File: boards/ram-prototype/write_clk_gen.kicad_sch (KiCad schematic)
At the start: 24 parts, among them U1 74LVC1G00, U2 74LVC1G00, U3 74LVC1G00, U4 74LVC1G00, U5 74LVC1G00, U6 74LVC1G00, U7 74LVC1G00, U8 74LVC1G00

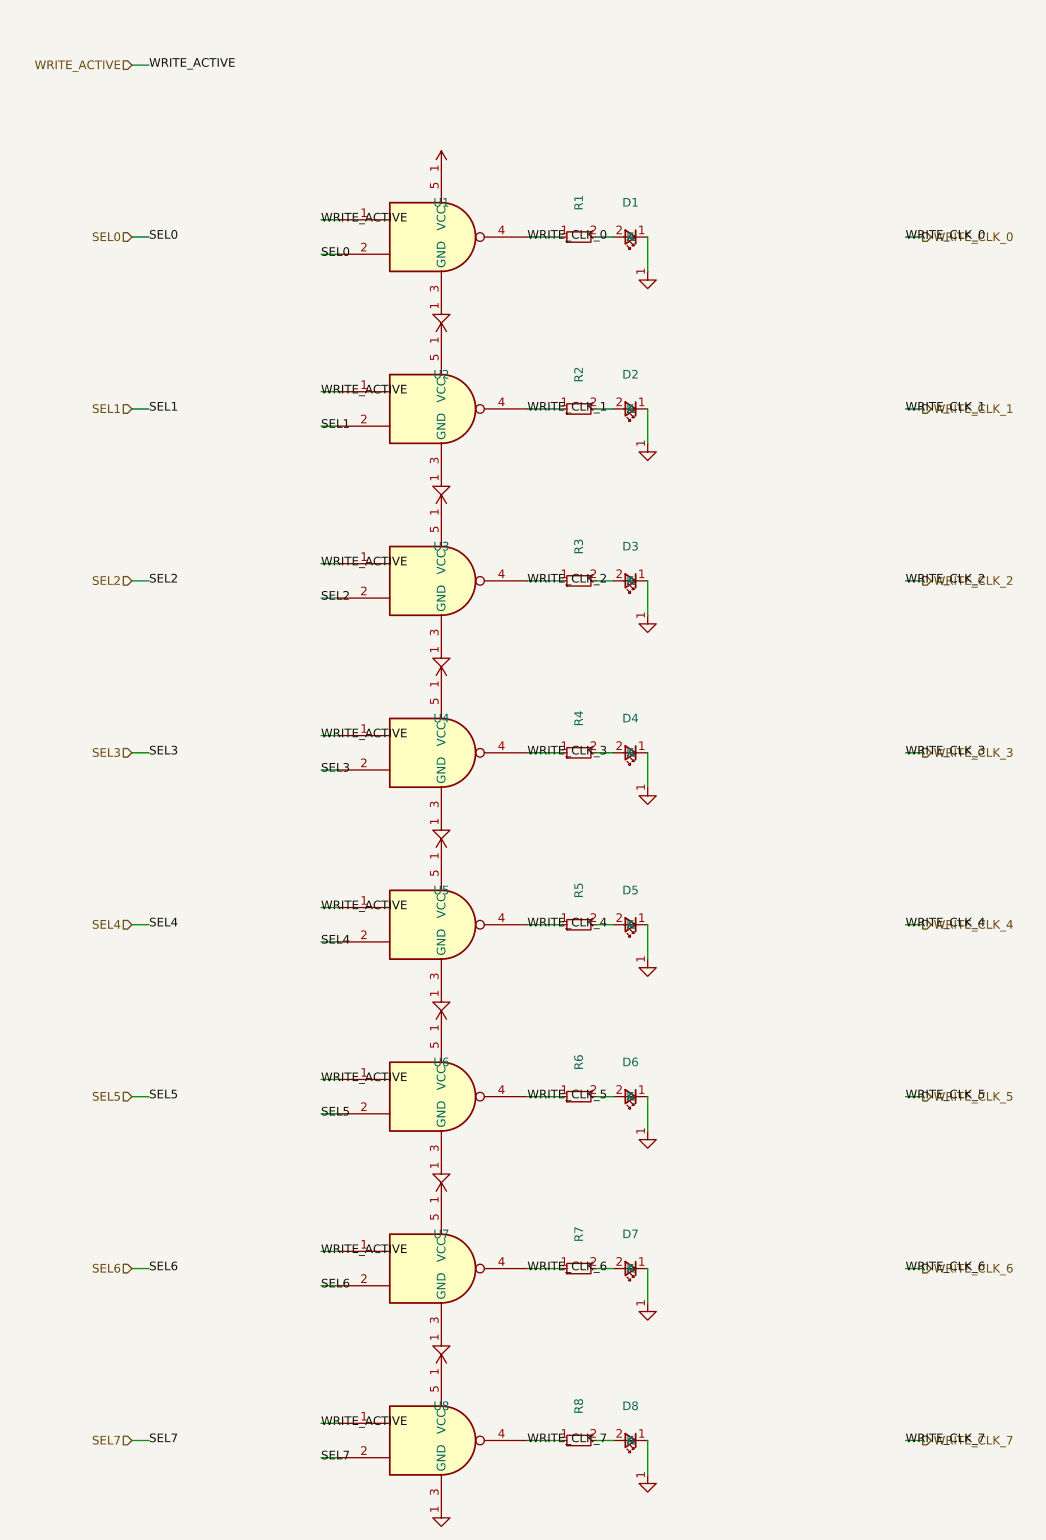
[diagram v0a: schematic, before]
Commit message: Schematic is starting to look good
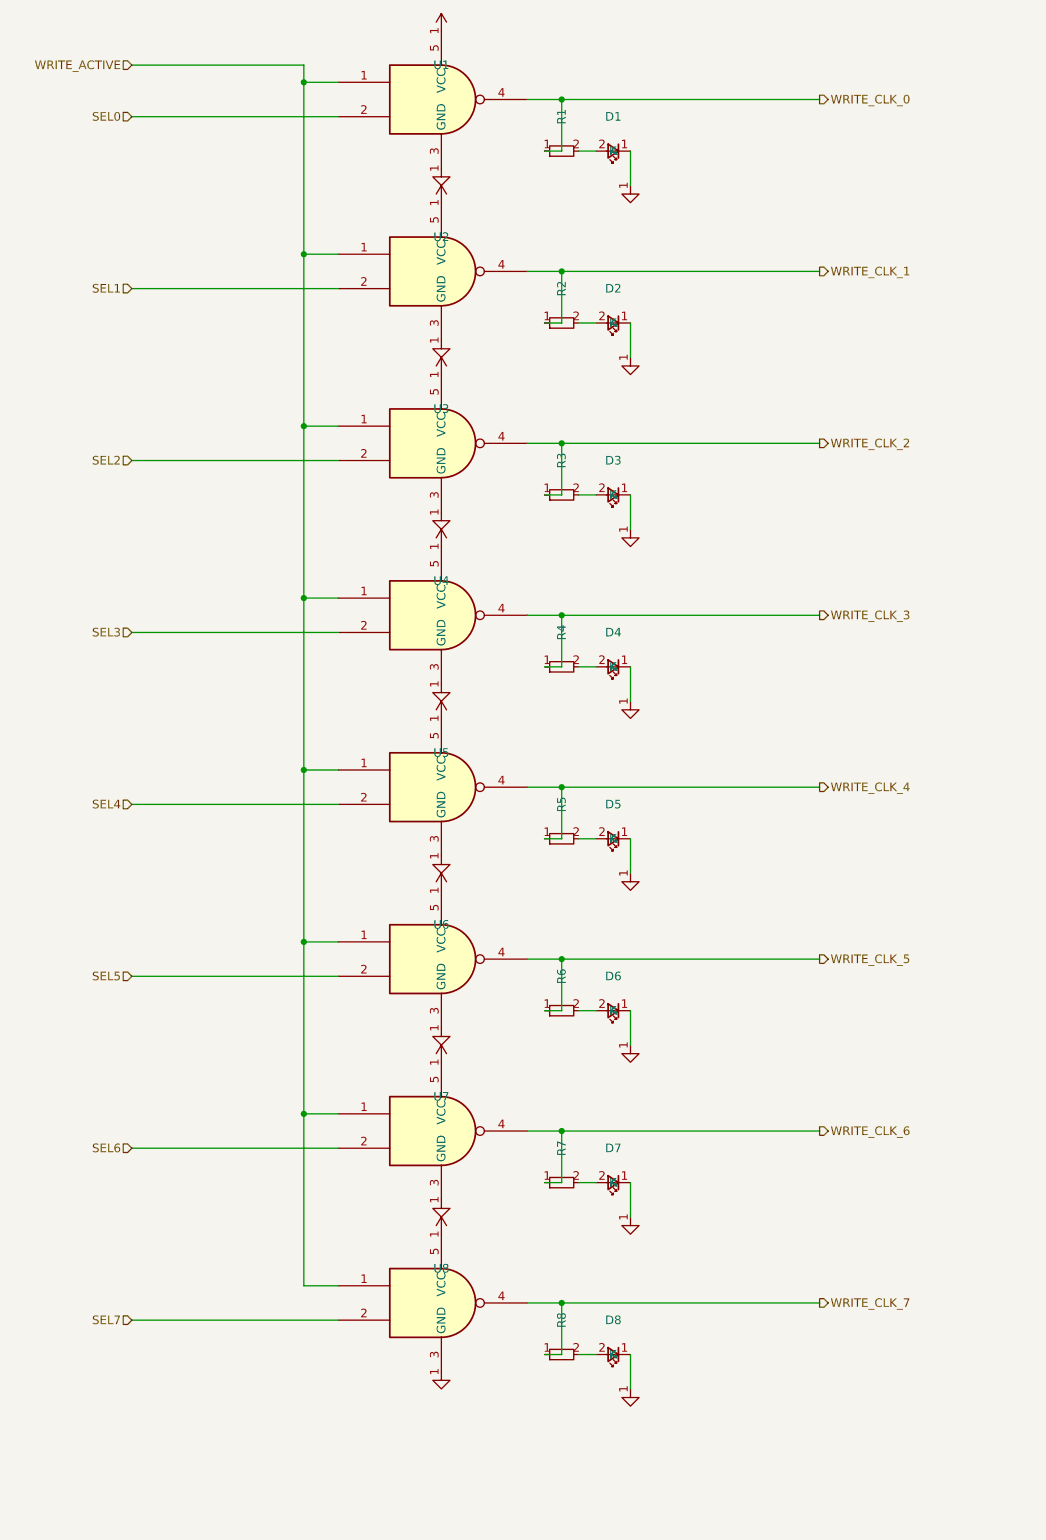
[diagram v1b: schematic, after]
